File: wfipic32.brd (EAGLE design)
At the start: 35.5 x 27.6 mm, 34 parts, among them IC1 BMA490L, J1 MLE-105-01-G-DV, J2 MLE-105-01-G-DV, J3 MLE-105-01-G-DV, J4 MLE-105-01-G-DV, U1 PIC32MK0512MCJ048T-I/Y8XTQFP4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, U2 MAX6126B30

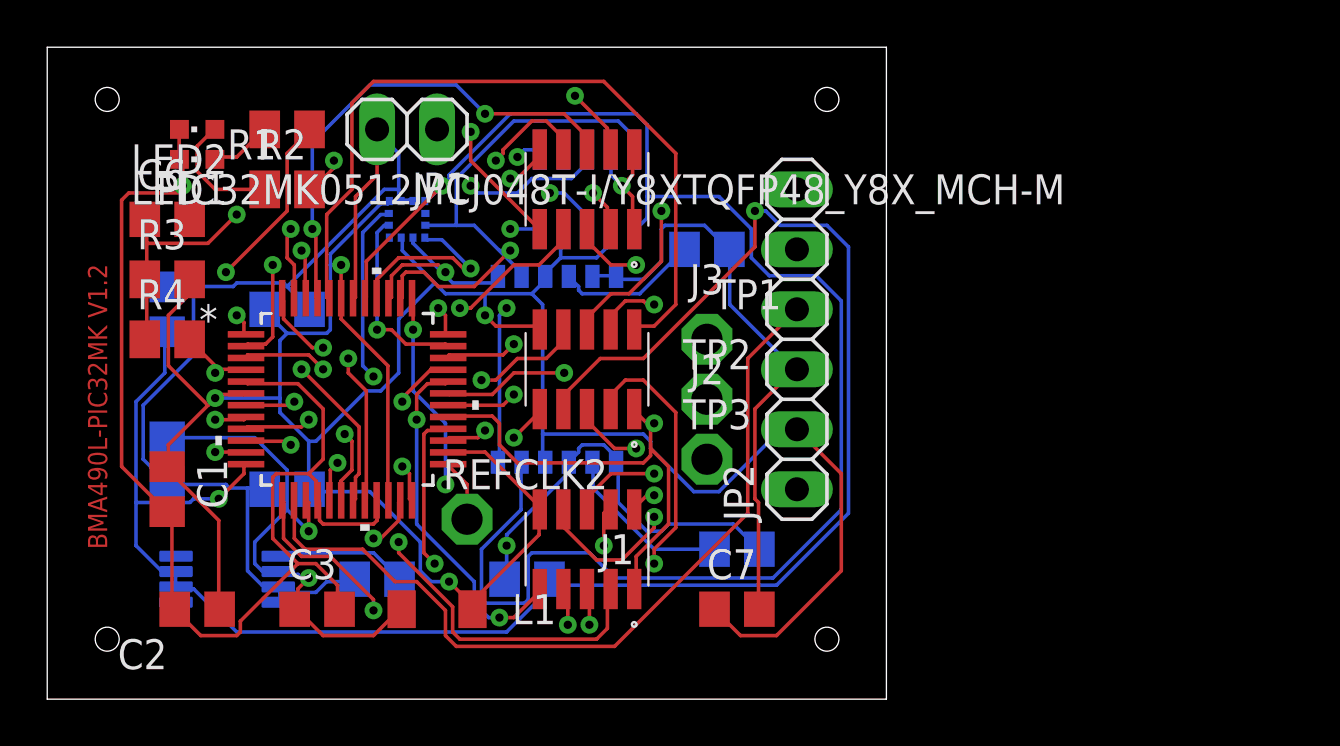
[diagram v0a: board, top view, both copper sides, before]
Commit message: up
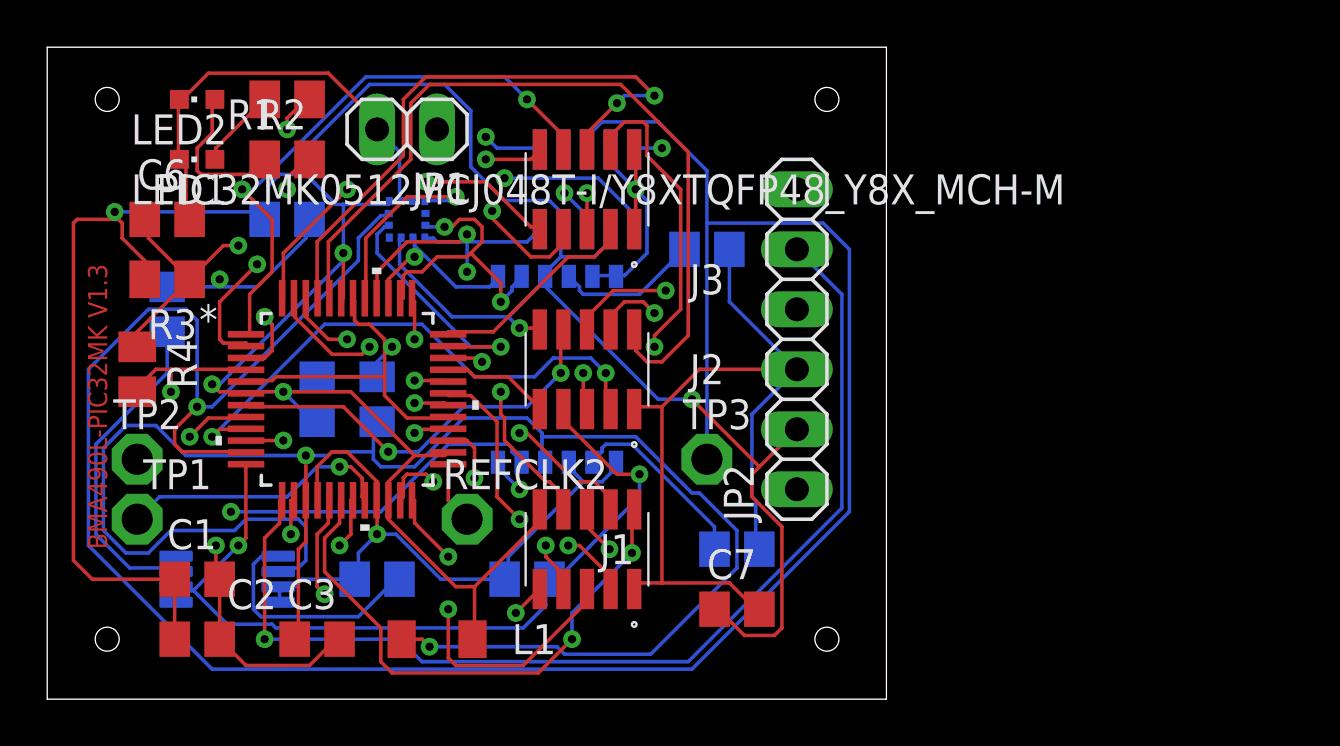
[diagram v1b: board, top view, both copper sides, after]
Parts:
- moved TP1 25.3 mm to (1.27, 35.6)
- moved TP2 24.3 mm to (1.27, 38.1)
- moved C10 9.25 mm to (11.4, 40.6), turned to 90 degrees
- moved C5 4.02 mm to (8.89, 40.6), turned to 90 degrees
- moved C1 4.02 mm to (3.81, 33.0), turned to 0 degrees
- moved C4 3.81 mm to (7.62, 48.3)
- moved R4 1.80 mm to (1.27, 41.9), turned to 270 degrees
- moved LED2 1.27 mm to (3.81, 53.3)
- moved R1 1.27 mm to (7.62, 53.3)
- moved C2 1.27 mm to (3.81, 30.5), turned to 0 degrees
- moved C3 1.27 mm to (8.89, 30.5)
- moved L1 1.27 mm to (14.0, 30.5)
- moved R2 1.27 mm to (7.62, 50.8)
- turned R3 to 180 degrees
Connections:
- net AVDD: now also AC1.4
- net VDD: no longer AC1.4
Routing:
- net BMA_INT2: track 51.0 -> 107.9 mm, vias 3 -> 1
- net AVDD: track 22.4 -> 75.3 mm
- net VSS: track 169.5 -> 131.3 mm, vias 4 -> 5
- net VREF+: track 78.8 -> 49.8 mm
- net PWM4ER: track 55.6 -> 27.1 mm
- net SDO1: track 34.1 -> 10.9 mm
- net IMU_CS: track 67.1 -> 48.9 mm, vias 1 -> 3
- net N$6: track 28.7 -> 12.3 mm
- net RED_LED: track 35.4 -> 19.1 mm
- net INDX2: track 36.2 -> 21.7 mm
- net PWM1L: track 18.5 -> 32.5 mm
- net SCK1: track 20.5 -> 9.29 mm
- net AN0: track 34.4 -> 23.3 mm
- net N$5: track 22.6 -> 11.6 mm
- net MCLR_SIG: track 35.7 -> 46.3 mm
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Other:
- board text added: "BMA490L-PIC32MK V1.3"
- board text removed: "BMA490L-PIC32MK V1.2"

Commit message: up
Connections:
- net PGC renamed PGC_C1RX
- net PGD renamed PGD_C1TX
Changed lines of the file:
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@@
 <via x="19.3675" y="49.37125" extent="1-16" drill="0.35"/>
 </signal>
-<signal name="PGD">
+<signal name="PGD_C1TX">
 <contactref element="JP2" pad="4"/>
 <contactref element="U1" pad="14"/>
@@
 <via x="7.77875" y="34.925" extent="1-16" drill="0.35"/>
 </signal>
-<signal name="PGC">
+<signal name="PGC_C1RX">
 <contactref element="JP2" pad="5"/>
 <contactref element="U1" pad="13"/>
